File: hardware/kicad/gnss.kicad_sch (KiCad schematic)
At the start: 11 parts, among them U11 TXB0106PWR, U7 L76L-M33

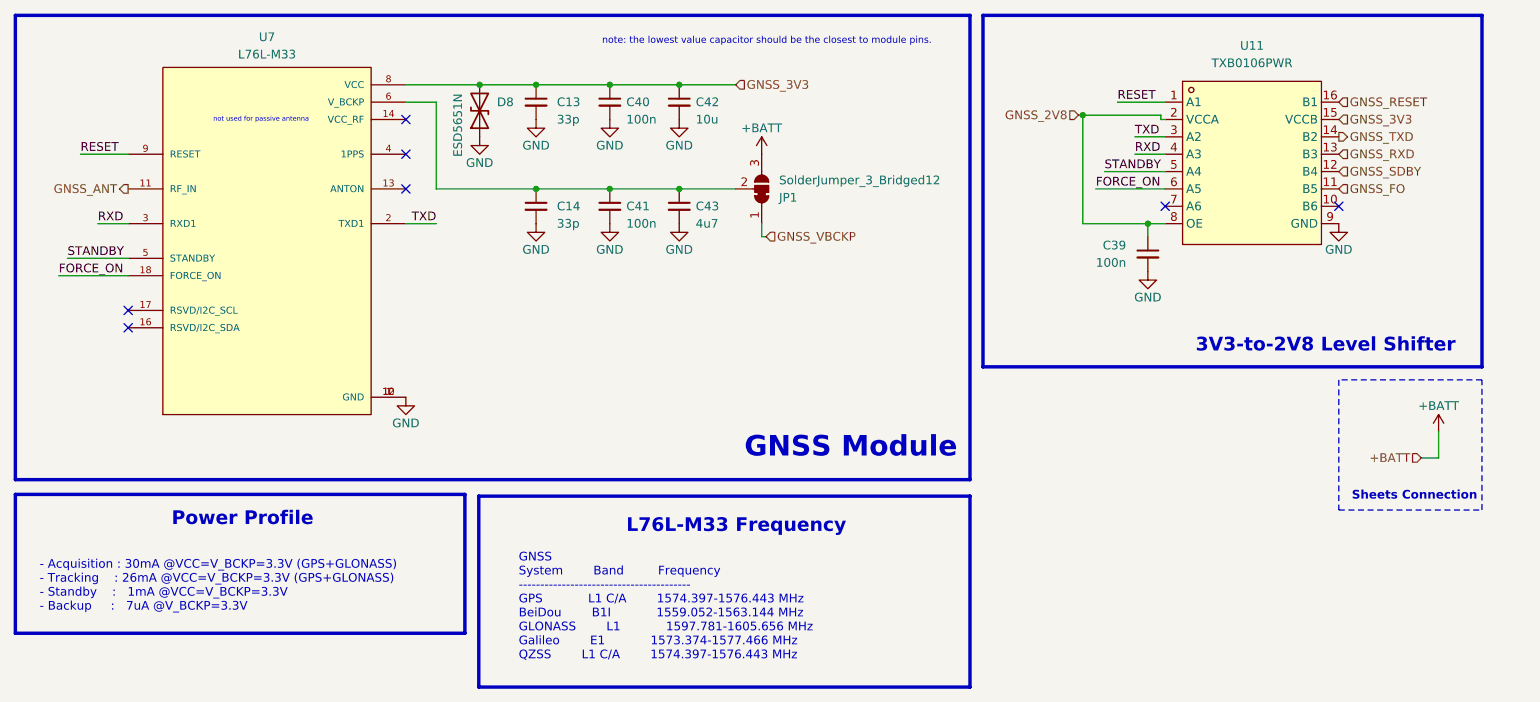
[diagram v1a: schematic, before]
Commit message: Start Rev 3
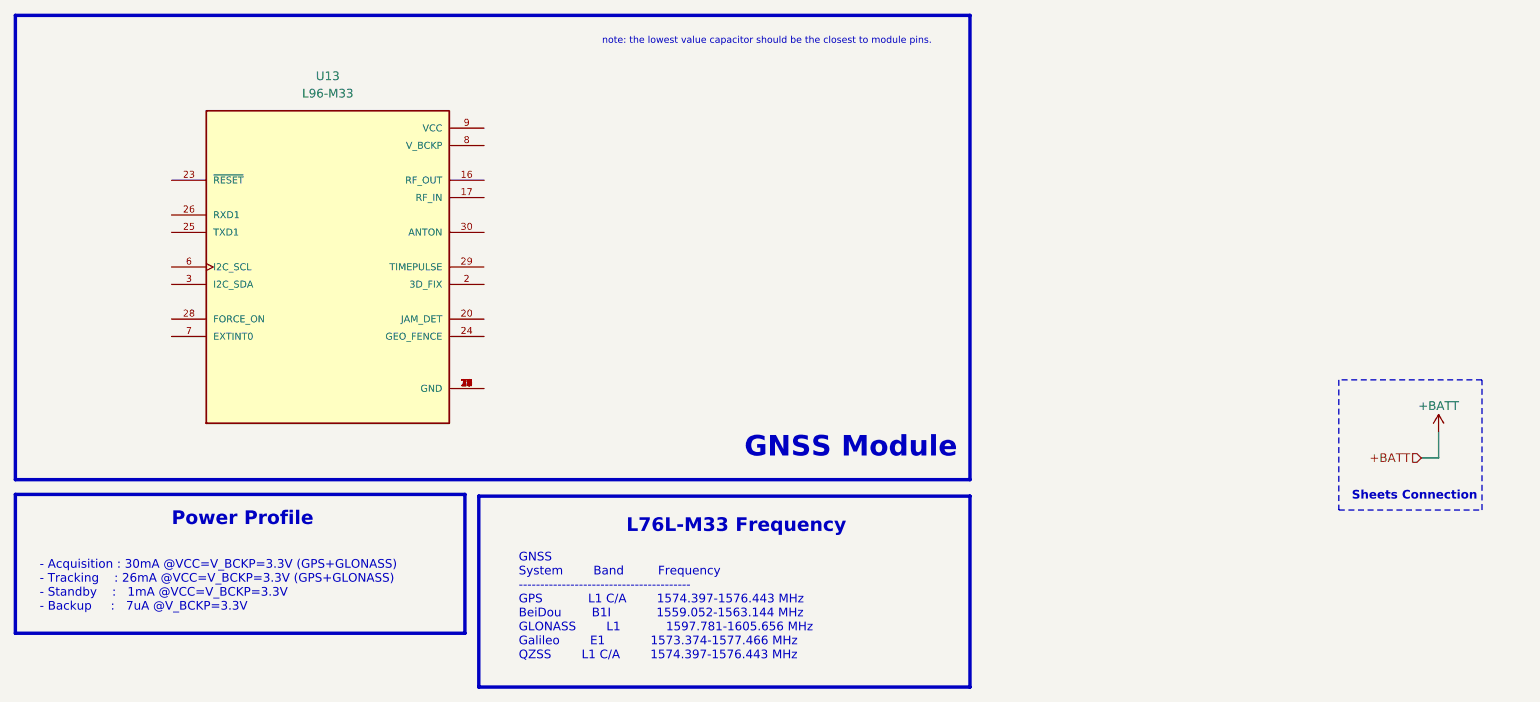
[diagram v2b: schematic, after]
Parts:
- removed C13, C14: 33p, Capacitor_SMD:C_0603_1608Metric, symbol Device:C_Small
- removed C39, C40, C41: 100n, Capacitor_SMD:C_0603_1608Metric, symbol Device:C_Small
- removed C42: 10u, Capacitor_SMD:C_0603_1608Metric, symbol Device:C_Small
- removed C43: 4u7, Capacitor_SMD:C_0603_1608Metric, symbol Device:C_Small
- removed D8: ESD5651N, Diode_SMD:D_SOD-882, symbol Device:D_TVS
- removed JP1: SolderJumper_3_Bridged12, Jumper:SolderJumper-3_P1.3mm_Bridged2Bar12_RoundedPad1.0x1.5mm, symbol Jumper:SolderJumper_3_Bridged12
- removed U11: TXB0106PWR, bwlc1a:TSSOP-16_L5.0-W4.4-P0.65-LS6.4-BL, symbol bwlc1a:TXB0106PWR
- removed U7: L76L-M33, bwlc1a:L76L-M33, symbol bwlc1a:L76L-M33
- added U13: L96-M33, bwlc1a:L96-M33, symbol bwlc1a:L96-M33
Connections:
- new net: U13.10 (GND), U13.11 (GND), U13.12 (GND), U13.13 (GND), U13.14 (GND), U13.15 (GND), U13.18 (GND), U13.19 (GND), U13.21 (GND), U13.22 (GND), U13.27 (GND), U13.31 (GND), U13.4 (GND), U13.5 (GND)
- no-connect marks 7 -> 0
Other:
- note removed: "3V3-to-2V8 Level Shifter"
- note removed: "not used for passive antenna"
